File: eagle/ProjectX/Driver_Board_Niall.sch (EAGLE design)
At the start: 13 parts, among them IC1 LM317MBSTT3

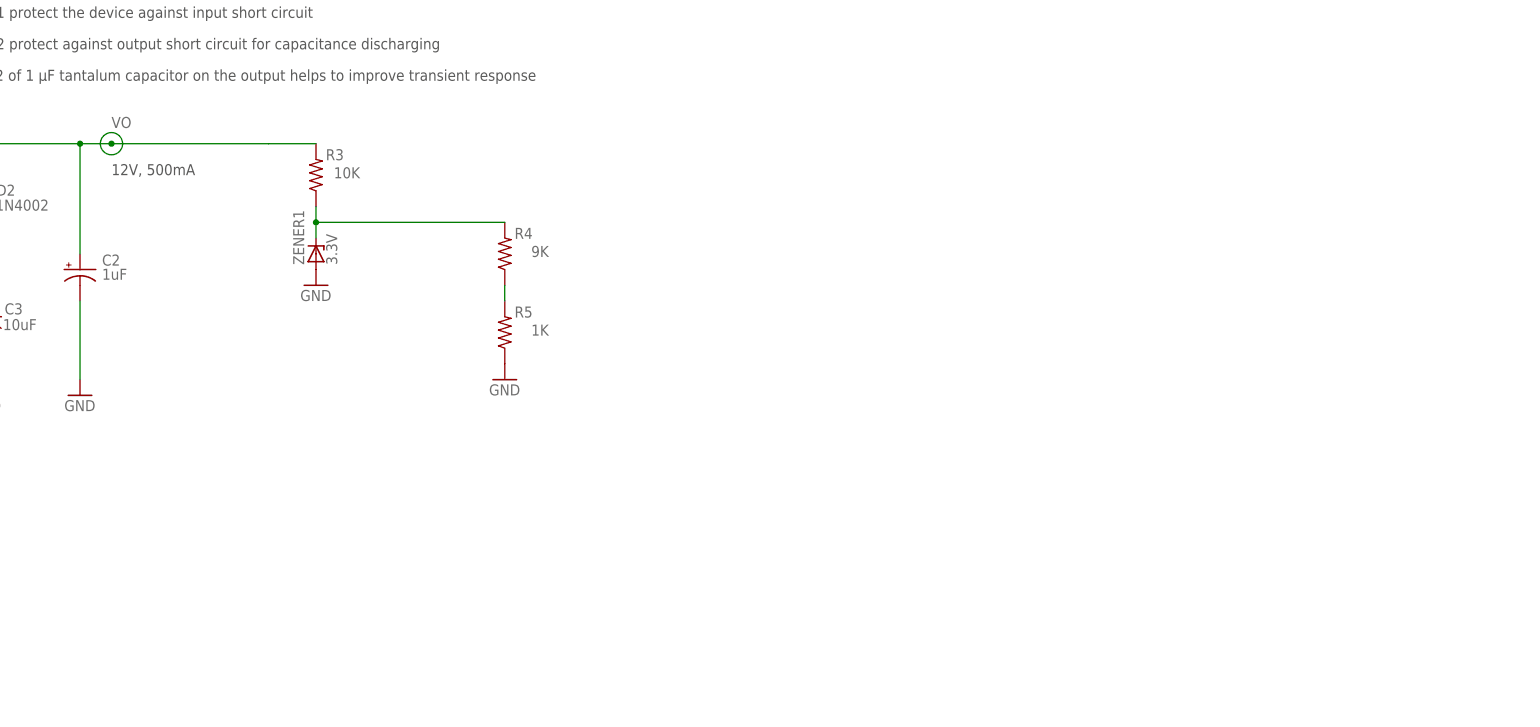
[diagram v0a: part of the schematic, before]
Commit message: Work in progress driver board
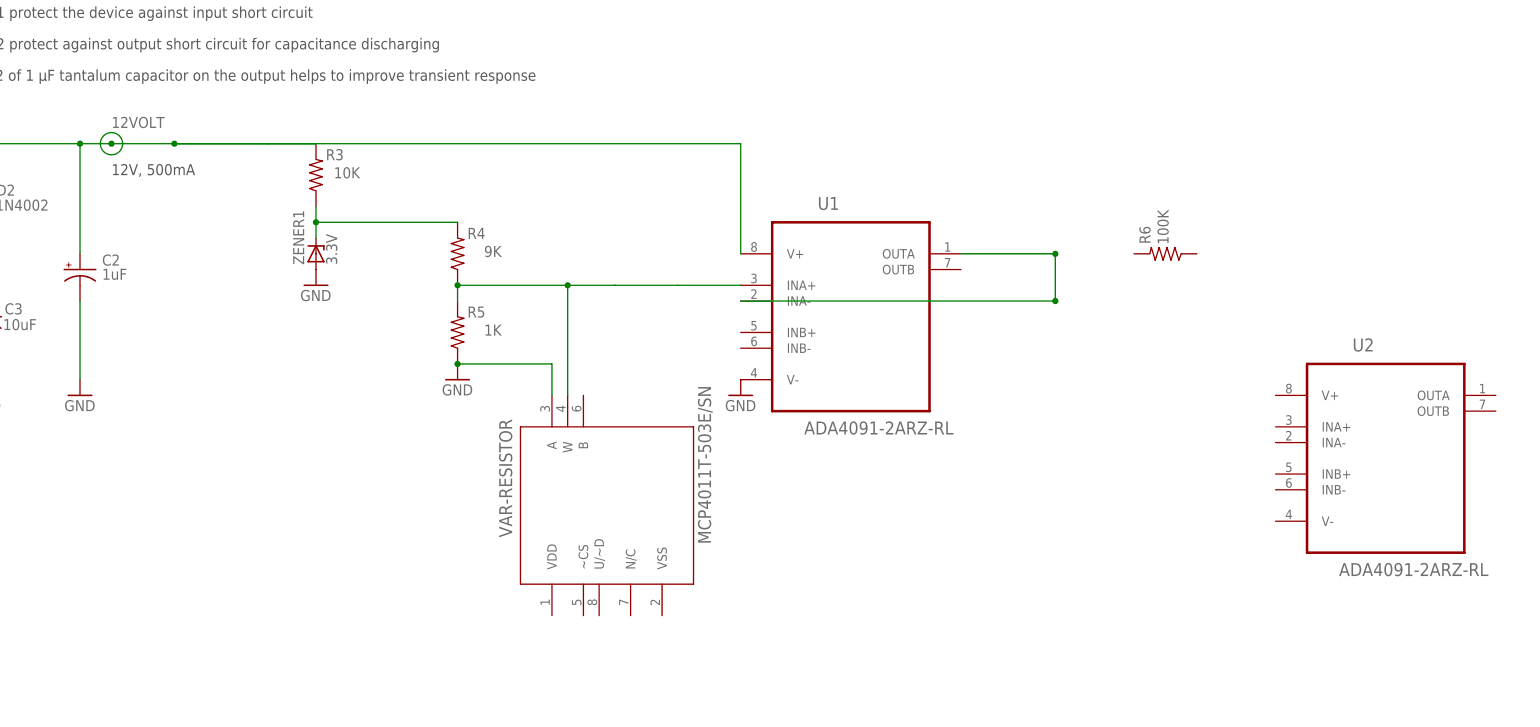
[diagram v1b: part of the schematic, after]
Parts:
- added R6: 100K, resistor:R-US_M0805
- added U1, U2: ADA4091-2ARZ-RL, SnapEDA-Library:ADA4091-2ARZ-RL
- added VAR-RESISTOR: MCP4011T-503E/SN, SnapEDA-Library:MCP4011T-503E/SN
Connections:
- removed net VO: C2.+, D1.A, D2.C, IC1.OUT, R1.2, R3.2
- new net 12VOLT: C2.+, D1.A, D2.C, IC1.OUT, R1.2, R3.2, U1.V+
- new net N$4: U1.INA-, U1.OUTA
- net GND: now also U1.V-, VAR-RESISTOR.A
- net N$2: now also U1.INA+, VAR-RESISTOR.W
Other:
- moved on the sheet: R4, R5
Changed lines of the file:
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@@
 <attribute name="PARTNUMBER" value="LM317M"/>
 </part>
-<part name="R1" library="resistor" library_urn="urn:adsk.eagle:library:348" deviceset="R-US_" device="M0805" package3d_urn="urn:adsk.eagle:package:26079/1" value="240Ω"/>
+<part name="R1" library="resistor" library_urn="urn:adsk.eagle:library:348" deviceset="R-US_" device="M0805" package3d_urn="urn:adsk.eagle:package:23556/1" value="240Ω"/>
 <part name="C1" library="rcl" library_urn="urn:adsk.eagle:library:334" deviceset="C-EU" device="075-052X106" package3d_urn="urn:adsk.eagle:package:23650/1" value="0.1uF"/>
-<part name="C2" library="resistor" library_urn="urn:adsk.eagle:library:348" deviceset="CPOL-US" device="085CS-1AR" package3d_urn="urn:adsk.eagle:package:25875/1" value="1uF"/>
-<part name="C3" library="resistor" library_urn="urn:adsk.eagle:library:348" deviceset="CPOL-US" device="085CS-1AR" package3d_urn="urn:adsk.eagle:package:25875/1" value="10uF"/>
+<part name="C2" library="resistor" library_urn="urn:adsk.eagle:library:348" deviceset="CPOL-US" device="085CS-1AR" package3d_urn="urn:adsk.eagle:package:23396/1" value="1uF"/>
+<part name="C3" library="resistor" library_urn="urn:adsk.eagle:library:348" deviceset="CPOL-US" device="085CS-1AR" package3d_urn="urn:adsk.eagle:package:23396/1" value="10uF"/>
 <part name="D1" library="diode" deviceset="1N4004" device="" package3d_urn="urn:adsk.eagle:package:43336/1" value="1N4002"/>
 <part name="D2" library="diode" deviceset="1N4004" device="" package3d_urn="urn:adsk.eagle:package:43336/1" value="1N4002"/>
 <part name="SUPPLY3" library="supply1" library_urn="urn:adsk.eagle:library:371" deviceset="GND" device=""/>
-<part name="R2" library="resistor" library_urn="urn:adsk.eagle:library:348" deviceset="R-US_" device="M0805" package3d_urn="urn:adsk.eagle:package:26079/1" value="2.1K"/>
+<part name="R2" library="resistor" library_urn="urn:adsk.eagle:library:348" deviceset="R-US_" device="M0805" package3d_urn="urn:adsk.eagle:package:23556/1" value="2.1K"/>
 <part name="SUPPLY1" library="supply1" library_urn="urn:adsk.eagle:library:371" deviceset="GND" device=""/>
 <part name="SUPPLY2" library="supply1" library_urn="urn:adsk.eagle:library:371" deviceset="GND" device=""/>
 <part name="SUPPLY4" library="supply1" library_urn="urn:adsk.eagle:library:371" deviceset="GND" device=""/>
-<part name="R3" library="resistor" library_urn="urn:adsk.eagle:library:348" deviceset="R-US_" device="M0805" package3d_urn="urn:adsk.eagle:package:26079/1" value="10K"/>
-<part name="R4" library="resistor" library_urn="urn:adsk.eagle:library:348" deviceset="R-US_" device="M0805" package3d_urn="urn:adsk.eagle:package:26079/1" value="9K"/>
-<part name="R5" library="resistor" library_urn="urn:adsk.eagle:library:348" deviceset="R-US_" device="M0805" package3d_urn="urn:adsk.eagle:package:26079/1" value="1K"/>
+<part name="R3" library="resistor" library_urn="urn:adsk.eagle:library:348" deviceset="R-US_" device="M0805" package3d_urn="urn:adsk.eagle:package:23556/1" value="10K"/>
+<part name="R4" library="resistor" library_urn="urn:adsk.eagle:library:348" deviceset="R-US_" device="M0805" package3d_urn="urn:adsk.eagle:package:23556/1" value="9K"/>
+<part name="R5" library="resistor" library_urn="urn:adsk.eagle:library:348" deviceset="R-US_" device="M0805" package3d_urn="urn:adsk.eagle:package:23556/1" value="1K"/>
 <part name="ZENER1" library="diode" library_urn="urn:adsk.eagle:library:210" deviceset="ZENER-DIODE" device="C1702-15" package3d_urn="urn:adsk.eagle:package:43351/1" value="3.3V"/>
 <part name="SUPPLY5" library="supply1" library_urn="urn:adsk.eagle:library:371" deviceset="GND" device=""/>
 <part name="SUPPLY6" library="supply1" library_urn="urn:adsk.eagle:library:371" deviceset="GND" device=""/>
 <part name="U$2" library="Teensy356" deviceset="TEENSY_3.5/3.6" device=""/>
+<part name="U1" library="SnapEDA-Library" deviceset="ADA4091-2ARZ-RL" device=""/>
+<part name="SUPPLY7" library="supply1" library_urn="urn:adsk.eagle:library:371" deviceset="GND" device=""/>
+<part name="U2" library="SnapEDA-Library" deviceset="ADA4091-2ARZ-RL" device=""/>
+<part name="R6" library="resistor" library_urn="urn:adsk.eagle:library:348" deviceset="R-US_" device="M0805" package3d_urn="urn:adsk.eagle:package:23556/1" value="100K"/>
+<part name="VAR-RESISTOR" library="SnapEDA-Library" deviceset="MCP4011T-503E/SN" device=""/>
 </parts>
 <sheets>
@@
 <attribute name="VALUE" x="50.292" y="179.07" size="1.778" layer="96" rot="R180"/>
 </instance>
-<instance part="R4" gate="G$1" x="73.66" y="165.1" smashed="yes" rot="R90">
-<attribute name="NAME" x="78.1614" y="169.29" size="1.778" layer="95" rot="R180"/>
-<attribute name="VALUE" x="80.772" y="166.37" size="1.778" layer="96" rot="R180"/>
-</instance>
-<instance part="R5" gate="G$1" x="73.66" y="152.4" smashed="yes" rot="R90">
-<attribute name="NAME" x="78.1614" y="156.59" size="1.778" layer="95" rot="R180"/>
-<attribute name="VALUE" x="80.772" y="153.67" size="1.778" layer="96" rot="R180"/>
+<instance part="R4" gate="G$1" x="66.04" y="165.1" smashed="yes" rot="R90">
+<attribute name="NAME" x="70.5414" y="169.29" size="1.778" layer="95" rot="R180"/>
+<attribute name="VALUE" x="73.152" y="166.37" size="1.778" layer="96" rot="R180"/>
+</instance>
+<instance part="R5" gate="G$1" x="66.04" y="152.4" smashed="yes" rot="R90">
+<attribute name="NAME" x="70.5414" y="156.59" size="1.778" layer="95" rot="R180"/>
+<attribute name="VALUE" x="73.152" y="153.67" size="1.778" layer="96" rot="R180"/>
 </instance>
 <instance part="ZENER1" gate="G$1" x="43.18" y="165.1" rot="R90"/>
 <instance part="SUPPLY5" gate="1" x="43.18" y="160.02"/>
-<instance part="SUPPLY6" gate="1" x="73.66" y="144.78"/>
+<instance part="SUPPLY6" gate="1" x="66.04" y="144.78"/>
 <instance part="U$2" gate="G$1" x="-38.1" y="96.52"/>
+<instance part="U1" gate="A" x="129.54" y="157.48"/>
+<instance part="SUPPLY7" gate="1" x="111.76" y="142.24"/>
+<instance part="U2" gate="A" x="215.9" y="134.62"/>
+<instance part="R6" gate="G$1" x="180.34" y="165.1" smashed="yes" rot="R180">
+<attribute name="NAME" x="176.15" y="169.6014" size="1.778" layer="95" rot="R270"/>
+<attribute name="VALUE" x="179.07" y="172.212" size="1.778" layer="96" rot="R270"/>
+</instance>
+<instance part="VAR-RESISTOR" gate="A" x="81.28" y="106.68" rot="R90"/>
 </instances>
 <busses>
@@
 <pinref part="R5" gate="G$1" pin="1"/>
 <pinref part="SUPPLY6" gate="1" pin="GND"/>
+<wire x1="66.04" y1="147.32" x2="81.28" y2="147.32" width="0.1524" layer="91"/>
+<junction x="66.04" y="147.32"/>
+<pinref part="VAR-RESISTOR" gate="A" pin="A"/>
+<wire x1="81.28" y1="147.32" x2="81.28" y2="142.24" width="0.1524" layer="91"/>
+</segment>
+<segment>
+<pinref part="U1" gate="A" pin="V-"/>
+<pinref part="SUPPLY7" gate="1" pin="GND"/>
 </segment>
 </net>
@@
 </segment>
 </net>
-<net name="VO" class="0">
+<net name="12VOLT" class="0">
 <segment>
 <pinref part="D2" gate="1" pin="C"/>
@@
 <junction x="10.16" y="182.88"/>
 <pinref part="R3" gate="G$1" pin="2"/>
-<wire x1="10.16" y1="182.88" x2="35.56" y2="182.88" width="0.1524" layer="91"/>
+<wire x1="10.16" y1="182.88" x2="20.32" y2="182.88" width="0.1524" layer="91"/>
+<wire x1="20.32" y1="182.88" x2="35.56" y2="182.88" width="0.1524" layer="91"/>
 <wire x1="35.56" y1="182.88" x2="43.18" y2="182.88" width="0.1524" layer="91"/>
+<pinref part="U1" gate="A" pin="V+"/>
+<wire x1="20.32" y1="182.88" x2="111.76" y2="182.88" width="0.1524" layer="91"/>
+<wire x1="111.76" y1="182.88" x2="111.76" y2="165.1" width="0.1524" layer="91"/>
+<junction x="20.32" y="182.88"/>
 </segment>
 </net>
@@
 <wire x1="43.18" y1="170.18" x2="43.18" y2="167.64" width="0.1524" layer="91"/>
 <pinref part="R4" gate="G$1" pin="2"/>
-<wire x1="43.18" y1="170.18" x2="73.66" y2="170.18" width="0.1524" layer="91"/>
+<wire x1="43.18" y1="170.18" x2="66.04" y2="170.18" width="0.1524" layer="91"/>
 <junction x="43.18" y="170.18"/>
 </segment>
@@
 <pinref part="R4" gate="G$1" pin="1"/>
 <pinref part="R5" gate="G$1" pin="2"/>
-<wire x1="73.66" y1="157.48" x2="73.66" y2="160.02" width="0.1524" layer="91"/>
+<wire x1="66.04" y1="157.48" x2="66.04" y2="160.02" width="0.1524" layer="91"/>
+<pinref part="U1" gate="A" pin="INA+"/>
+<wire x1="66.04" y1="160.02" x2="83.82" y2="160.02" width="0.1524" layer="91"/>
+<wire x1="83.82" y1="160.02" x2="91.44" y2="160.02" width="0.1524" layer="91"/>
+<wire x1="91.44" y1="160.02" x2="101.6" y2="160.02" width="0.1524" layer="91"/>
+<wire x1="101.6" y1="160.02" x2="111.76" y2="160.02" width="0.1524" layer="91"/>
+<junction x="66.04" y="160.02"/>
+<pinref part="VAR-RESISTOR" gate="A" pin="W"/>
+<wire x1="83.82" y1="142.24" x2="83.82" y2="160.02" width="0.1524" layer="91"/>
+<junction x="83.82" y="160.02"/>
+</segment>
+</net>
+<net name="N$4" class="0">
+<segment>
+<pinref part="U1" gate="A" pin="OUTA"/>
+<pinref part="U1" gate="A" pin="INA-"/>
+<wire x1="147.32" y1="165.1" x2="162.56" y2="165.1" width="0.1524" layer="91"/>
+<wire x1="162.56" y1="165.1" x2="162.56" y2="157.48" width="0.1524" layer="91"/>
+<junction x="162.56" y="165.1"/>
+<junction x="162.56" y="157.48"/>
+<wire x1="162.56" y1="157.48" x2="111.76" y2="157.48" width="0.1524" layer="91"/>
 </segment>
 </net>
@@
 packages will not be understood (or retained) with this version.
 </note>
+<note version="8.4" severity="warning">
+Since Version 8.4, EAGLE supports properties for SPICE simulation.
+Probes in schematics and SPICE mapping objects found in parts and library devices
+will not be understood with this version. Update EAGLE to the latest version
+for full support of SPICE simulation.
+</note>
 </compatibility>
